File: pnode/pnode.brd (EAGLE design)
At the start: 50 x 23 mm, 39 parts, among them IC2 HTU21D, IC3 SI4012

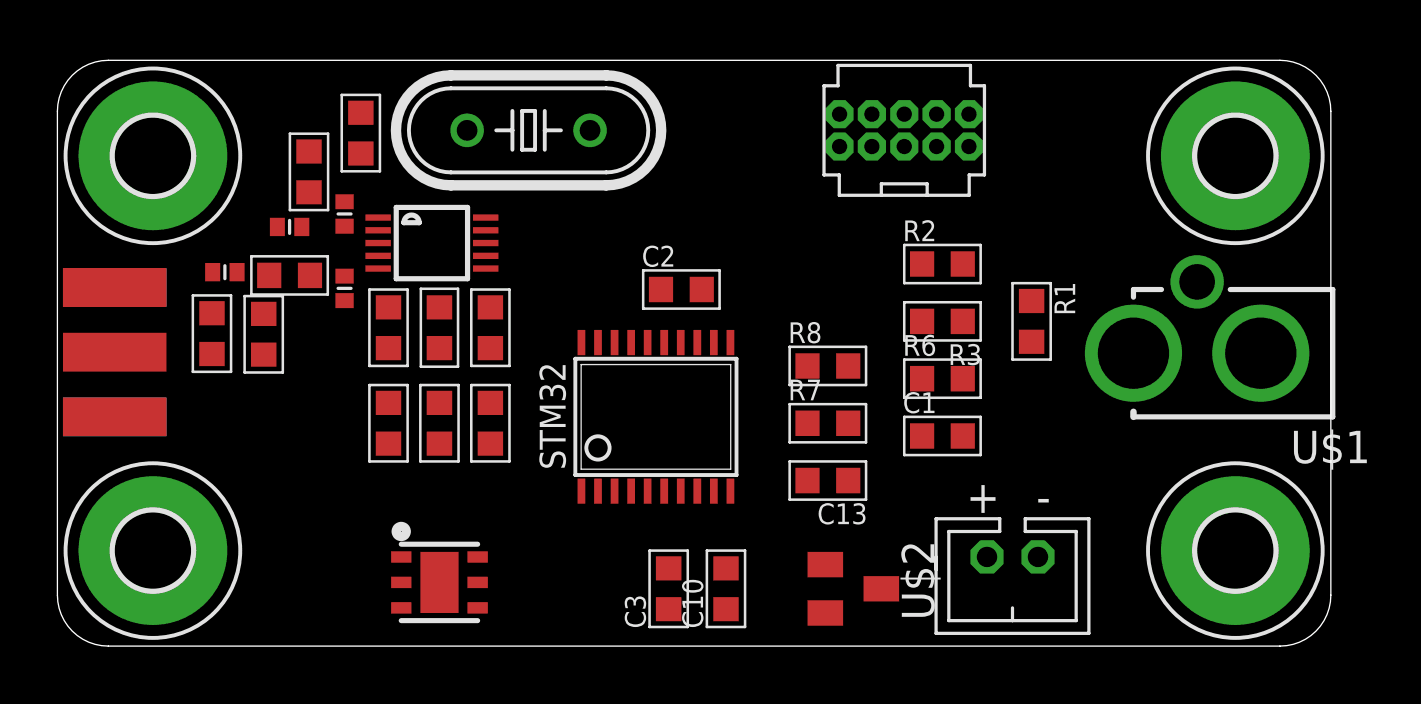
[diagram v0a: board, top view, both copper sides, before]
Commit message: routing pnode
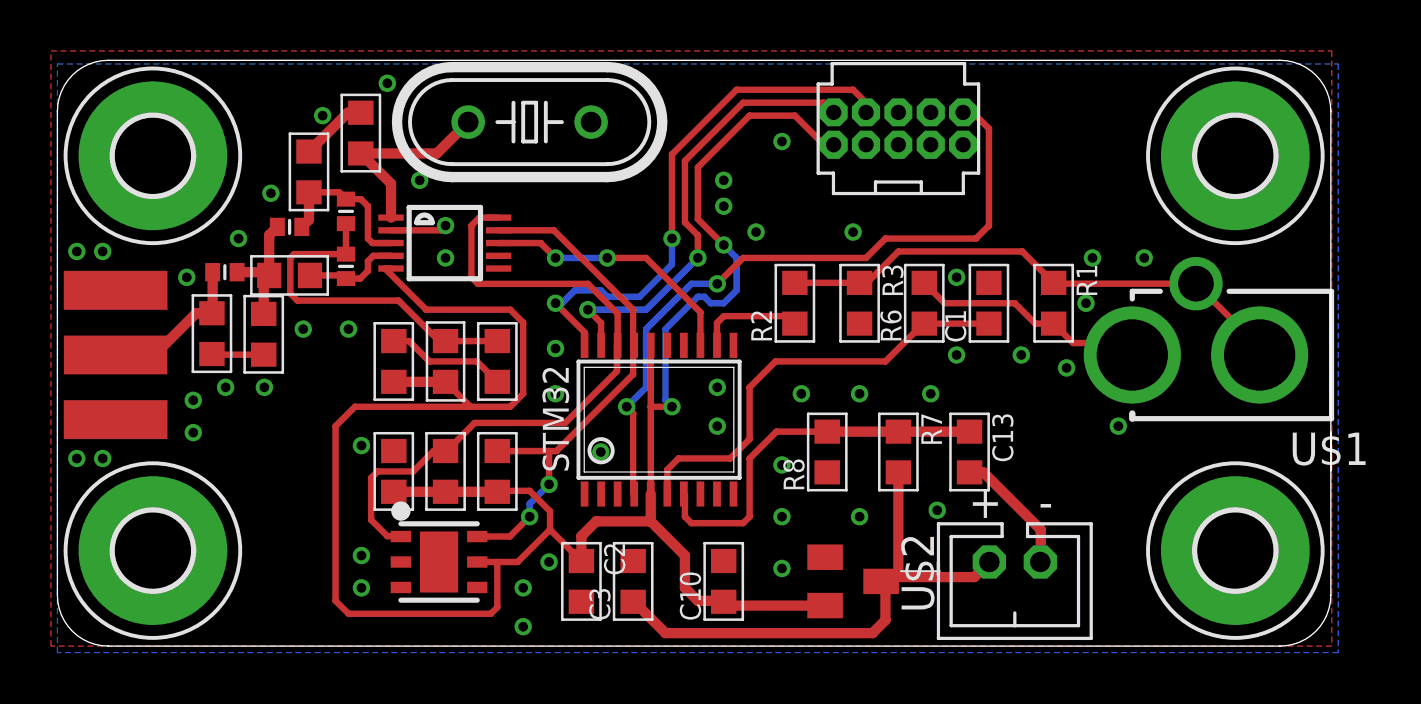
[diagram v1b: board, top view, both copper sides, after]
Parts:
- moved C2 12.1 mm to (20.6, 2.54), turned to 270 degrees
- moved R2 5.99 mm to (29.0, 13.5), turned to 90 degrees
- moved C13 5.68 mm to (35.8, 7.62), turned to 270 degrees
- moved C1 5.52 mm to (36.6, 13.5), turned to 90 degrees
- moved R8 3.38 mm to (30.2, 7.62), turned to 90 degrees
- moved R3 3.33 mm to (31.5, 13.5), turned to 270 degrees
- moved R6 3.05 mm to (34.0, 13.5), turned to 90 degrees
- moved R7 2.99 mm to (33.0, 7.62), turned to 270 degrees
- moved R5 1.91 mm to (17.3, 6.86)
- moved R4 1.91 mm to (15.2, 6.86)
- moved C4 1.90 mm to (13.2, 6.86), turned to 90 degrees
- moved C3 1.42 mm to (22.6, 2.54)
- moved C8 1.35 mm to (17.3, 11.2)
- moved L1 1.35 mm to (15.2, 11.2)
- moved C7 1.34 mm to (13.2, 11.2), turned to 90 degrees
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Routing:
- net +3V3: track 0.00 -> 87.8 mm, vias 0 -> 2
- net NRST: track 0.00 -> 27.1 mm, vias 0 -> 2
- net SDA: track 0.00 -> 26.3 mm
- net SWCLK: track 0.00 -> 21.1 mm, vias 0 -> 2
- net SCL: track 0.00 -> 21.0 mm, vias 0 -> 2
- net VBATT: track 0.00 -> 20.9 mm
- net N$2: track 0.00 -> 20.6 mm
- net SWDAT: track 0.00 -> 17.7 mm, vias 0 -> 2
- net CLAMP: track 0.00 -> 17.2 mm
- net GND: track 0.00 -> 16.7 mm, vias 0 -> 50
- net VBATT_MEAS: track 0.00 -> 15.0 mm
- net N$4: track 0.00 -> 13.7 mm
- net RADIO_SHDN: track 0.00 -> 10.3 mm, vias 0 -> 2
- net N$1: track 0.00 -> 9.34 mm
- net N$5: track 0.00 -> 7.73 mm
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- added copper zone on layer 1, net GND
- added copper zone on layer 16, net GND

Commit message: Routing and tidying + silk
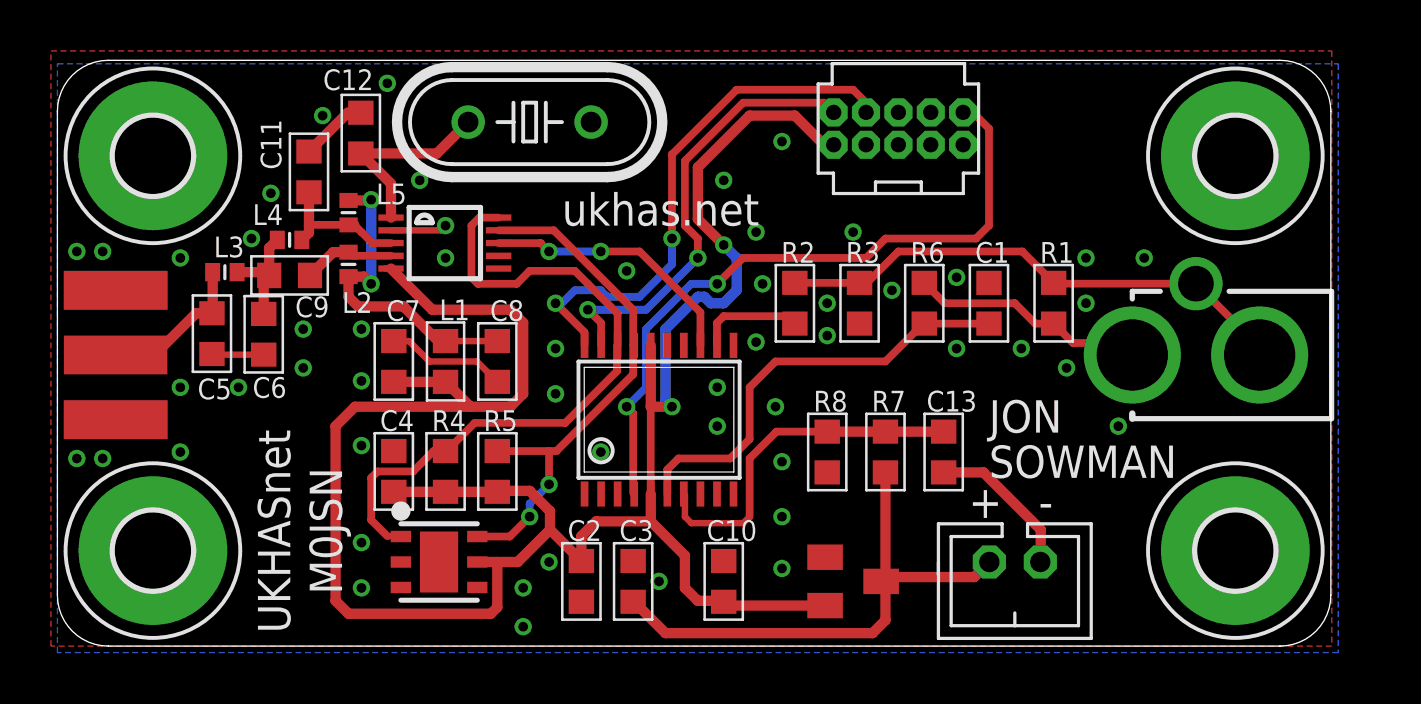
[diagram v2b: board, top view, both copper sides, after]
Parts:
- moved C13 1.02 mm to (34.8, 7.62)
- moved R7 0.51 mm to (32.5, 7.62)
- moved L4 0.51 mm to (9.12, 16.0)
- moved L2 0.12 mm to (11.4, 15.0), turned to 270 degrees
- moved L5 0.11 mm to (11.4, 17.0), turned to 90 degrees
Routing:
- net VBATT_MEAS: track 15.0 -> 14.0 mm
- net GND: track 16.7 -> 17.7 mm, vias 50 -> 53
- net N$4: track 13.7 -> 12.8 mm, vias 0 -> 2
- net N$8: track 6.27 -> 5.51 mm
- net N$7: track 4.95 -> 4.44 mm
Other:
- board text added: "JON"
- board text added: "M0JSN"
- board text added: "SOWMAN"
- board text added: "UKHASnet"
- board text added: "ukhas.net"
